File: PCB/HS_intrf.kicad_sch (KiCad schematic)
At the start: 17 parts, among them J801 USB4215-03-A_REVA, U301 STM32MP157FABx, U801 FUSB302BMPX, U802 HSP051-4M10

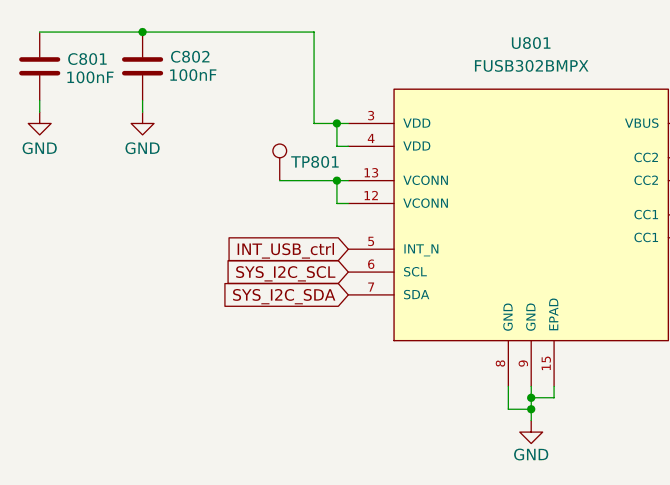
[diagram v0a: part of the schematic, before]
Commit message: pcb_update
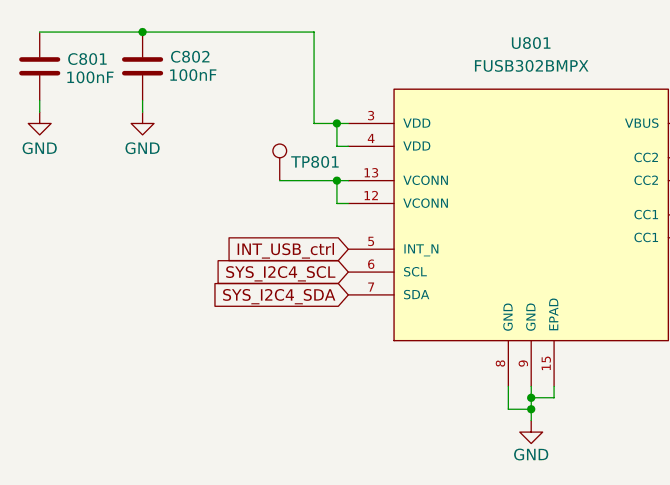
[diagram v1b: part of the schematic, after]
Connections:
- net SYS_I2C_SCL renamed SYS_I2C4_SCL
- net SYS_I2C_SDA renamed SYS_I2C4_SDA
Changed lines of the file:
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@@
 		)
 	)
-	(global_label "SYS_I2C_SDA"
+	(global_label "SYS_I2C4_SDA"
 		(shape input)
 		(at 62.23 167.64 180)
@@
 		)
 		(property "Intersheetrefs" "${INTERSHEET_REFS}"
-			(at 47.1496 167.64 0)
+			(at 45.9401 167.64 0)
 			(effects
 				(font
@@
 		)
 	)
-	(global_label "SYS_I2C_SCL"
+	(global_label "SYS_I2C4_SCL"
 		(shape input)
 		(at 62.23 165.1 180)
@@
 		)
 		(property "Intersheetrefs" "${INTERSHEET_REFS}"
-			(at 47.2101 165.1 0)
-			(effects
-				(font
+			(at 46.0006 165.1 0)
+			(effects
+				(font
